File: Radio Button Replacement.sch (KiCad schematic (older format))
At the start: 19 parts, among them SW1 SW_Push_SPDT_1_3_2, SW2 SW_Push_SPDT_1_3_2, SW3 SW_Push_SPDT_1_3_2, SW4 SW_Push_SPDT_1_3_2

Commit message: Center marks added
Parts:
- L1: Description (none) -> None; Manufacturer Name (none) -> None; Manufacturer Part No. (none) -> None; Source (none) -> None
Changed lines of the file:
@@
 F 1 "Logo" H 7135 6255 50  0000 L CNN
 F 2 "Logos:OSHW-Logo2_7.3x6mm_SilkScreen" H 7050 6300 50  0001 C CNN
-F 3 "" H 7050 6300 50  0001 C CNN
+F 3 "None" H 7050 6300 50  0001 C CNN
+F 4 "None" H 7050 6300 50  0001 C CNN "Description"
+F 5 "None" H 7050 6300 50  0001 C CNN "Manufacturer Name"
+F 6 "None" H 7050 6300 50  0001 C CNN "Manufacturer Part No."
+F 7 "None" H 7050 6300 50  0001 C CNN "Source"
 	1    7050 6300
 	1    0    0    -1

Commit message: Update resistor sizes
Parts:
- R1, R2, R3, R4, R5, R6, R7, R8: footprint Resistor_THT:R_Axial_DIN0204_L3.6mm_D1.6mm_P5.08mm_Horizontal -> Resistor_THT:R_Axial_DIN0204_L3.6mm_D1.6mm_P7.62mm_Horizontal
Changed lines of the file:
@@
 F 0 "R1" V 5500 3100 50  0000 C CNN
 F 1 "2.2k" V 5700 3100 50  0000 C CNN
-F 2 "Resistor_THT:R_Axial_DIN0204_L3.6mm_D1.6mm_P5.08mm_Horizontal" V 5530 3100 50  0001 C CNN
+F 2 "Resistor_THT:R_Axial_DIN0204_L3.6mm_D1.6mm_P7.62mm_Horizontal" V 5530 3100 50  0001 C CNN
 F 3 "https://www.seielect.com/catalog/sei-rnf_rnmf.pdf" H 5600 3100 50  0001 C CNN
 F 4 "2.2 kOhms ±1% 0.25W, 1/4W Through Hole Resistor Axial Flame Retardant Coating, Safety Metal Film" H 5600 3100 50  0001 C CNN "Description"
@@
 F 0 "R4" V 7200 3200 50  0000 C CNN
 F 1 "2.2k" V 7400 3200 50  0000 C CNN
-F 2 "Resistor_THT:R_Axial_DIN0204_L3.6mm_D1.6mm_P5.08mm_Horizontal" V 7230 3200 50  0001 C CNN
+F 2 "Resistor_THT:R_Axial_DIN0204_L3.6mm_D1.6mm_P7.62mm_Horizontal" V 7230 3200 50  0001 C CNN
 F 3 "https://www.seielect.com/catalog/sei-rnf_rnmf.pdf" H 7300 3200 50  0001 C CNN
 F 4 "2.2 kOhms ±1% 0.25W, 1/4W Through Hole Resistor Axial Flame Retardant Coating, Safety Metal Film" H 7300 3200 50  0001 C CNN "Description"
@@
 F 0 "R2" V 6050 2550 50  0000 C CNN
 F 1 "2.2k" V 6250 2550 50  0000 C CNN
-F 2 "Resistor_THT:R_Axial_DIN0204_L3.6mm_D1.6mm_P5.08mm_Horizontal" V 6080 2550 50  0001 C CNN
+F 2 "Resistor_THT:R_Axial_DIN0204_L3.6mm_D1.6mm_P7.62mm_Horizontal" V 6080 2550 50  0001 C CNN
 F 3 "https://www.seielect.com/catalog/sei-rnf_rnmf.pdf" H 6150 2550 50  0001 C CNN
 F 4 "2.2 kOhms ±1% 0.25W, 1/4W Through Hole Resistor Axial Flame Retardant Coating, Safety Metal Film" H 6150 2550 50  0001 C CNN "Description"
@@
 F 0 "R3" V 6650 2550 50  0000 C CNN
 F 1 "2.2k" V 6850 2550 50  0000 C CNN
-F 2 "Resistor_THT:R_Axial_DIN0204_L3.6mm_D1.6mm_P5.08mm_Horizontal" V 6680 2550 50  0001 C CNN
+F 2 "Resistor_THT:R_Axial_DIN0204_L3.6mm_D1.6mm_P7.62mm_Horizontal" V 6680 2550 50  0001 C CNN
 F 3 "https://www.seielect.com/catalog/sei-rnf_rnmf.pdf" H 6750 2550 50  0001 C CNN
 F 4 "2.2 kOhms ±1% 0.25W, 1/4W Through Hole Resistor Axial Flame Retardant Coating, Safety Metal Film" H 6750 2550 50  0001 C CNN "Description"
@@
 F 0 "R5" V 5500 4550 50  0000 C CNN
 F 1 "2.2k" V 5700 4550 50  0000 C CNN
-F 2 "Resistor_THT:R_Axial_DIN0204_L3.6mm_D1.6mm_P5.08mm_Horizontal" V 5530 4550 50  0001 C CNN
+F 2 "Resistor_THT:R_Axial_DIN0204_L3.6mm_D1.6mm_P7.62mm_Horizontal" V 5530 4550 50  0001 C CNN
 F 3 "https://www.seielect.com/catalog/sei-rnf_rnmf.pdf" H 5600 4550 50  0001 C CNN
 F 4 "2.2 kOhms ±1% 0.25W, 1/4W Through Hole Resistor Axial Flame Retardant Coating, Safety Metal Film" H 5600 4550 50  0001 C CNN "Description"
@@
 F 0 "R8" V 7200 4650 50  0000 C CNN
 F 1 "2.2k" V 7400 4650 50  0000 C CNN
-F 2 "Resistor_THT:R_Axial_DIN0204_L3.6mm_D1.6mm_P5.08mm_Horizontal" V 7230 4650 50  0001 C CNN
+F 2 "Resistor_THT:R_Axial_DIN0204_L3.6mm_D1.6mm_P7.62mm_Horizontal" V 7230 4650 50  0001 C CNN
 F 3 "https://www.seielect.com/catalog/sei-rnf_rnmf.pdf" H 7300 4650 50  0001 C CNN
 F 4 "2.2 kOhms ±1% 0.25W, 1/4W Through Hole Resistor Axial Flame Retardant Coating, Safety Metal Film" H 7300 4650 50  0001 C CNN "Description"
@@
 F 0 "R6" V 6050 4000 50  0000 C CNN
 F 1 "2.2k" V 6250 4000 50  0000 C CNN
-F 2 "Resistor_THT:R_Axial_DIN0204_L3.6mm_D1.6mm_P5.08mm_Horizontal" V 6080 4000 50  0001 C CNN
+F 2 "Resistor_THT:R_Axial_DIN0204_L3.6mm_D1.6mm_P7.62mm_Horizontal" V 6080 4000 50  0001 C CNN
 F 3 "https://www.seielect.com/catalog/sei-rnf_rnmf.pdf" H 6150 4000 50  0001 C CNN
 F 4 "2.2 kOhms ±1% 0.25W, 1/4W Through Hole Resistor Axial Flame Retardant Coating, Safety Metal Film" H 6150 4000 50  0001 C CNN "Description"
@@
 F 0 "R7" V 6650 4000 50  0000 C CNN
 F 1 "2.2k" V 6850 4000 50  0000 C CNN
-F 2 "Resistor_THT:R_Axial_DIN0204_L3.6mm_D1.6mm_P5.08mm_Horizontal" V 6680 4000 50  0001 C CNN
+F 2 "Resistor_THT:R_Axial_DIN0204_L3.6mm_D1.6mm_P7.62mm_Horizontal" V 6680 4000 50  0001 C CNN
 F 3 "https://www.seielect.com/catalog/sei-rnf_rnmf.pdf" H 6750 4000 50  0001 C CNN
 F 4 "2.2 kOhms ±1% 0.25W, 1/4W Through Hole Resistor Axial Flame Retardant Coating, Safety Metal Film" H 6750 4000 50  0001 C CNN "Description"

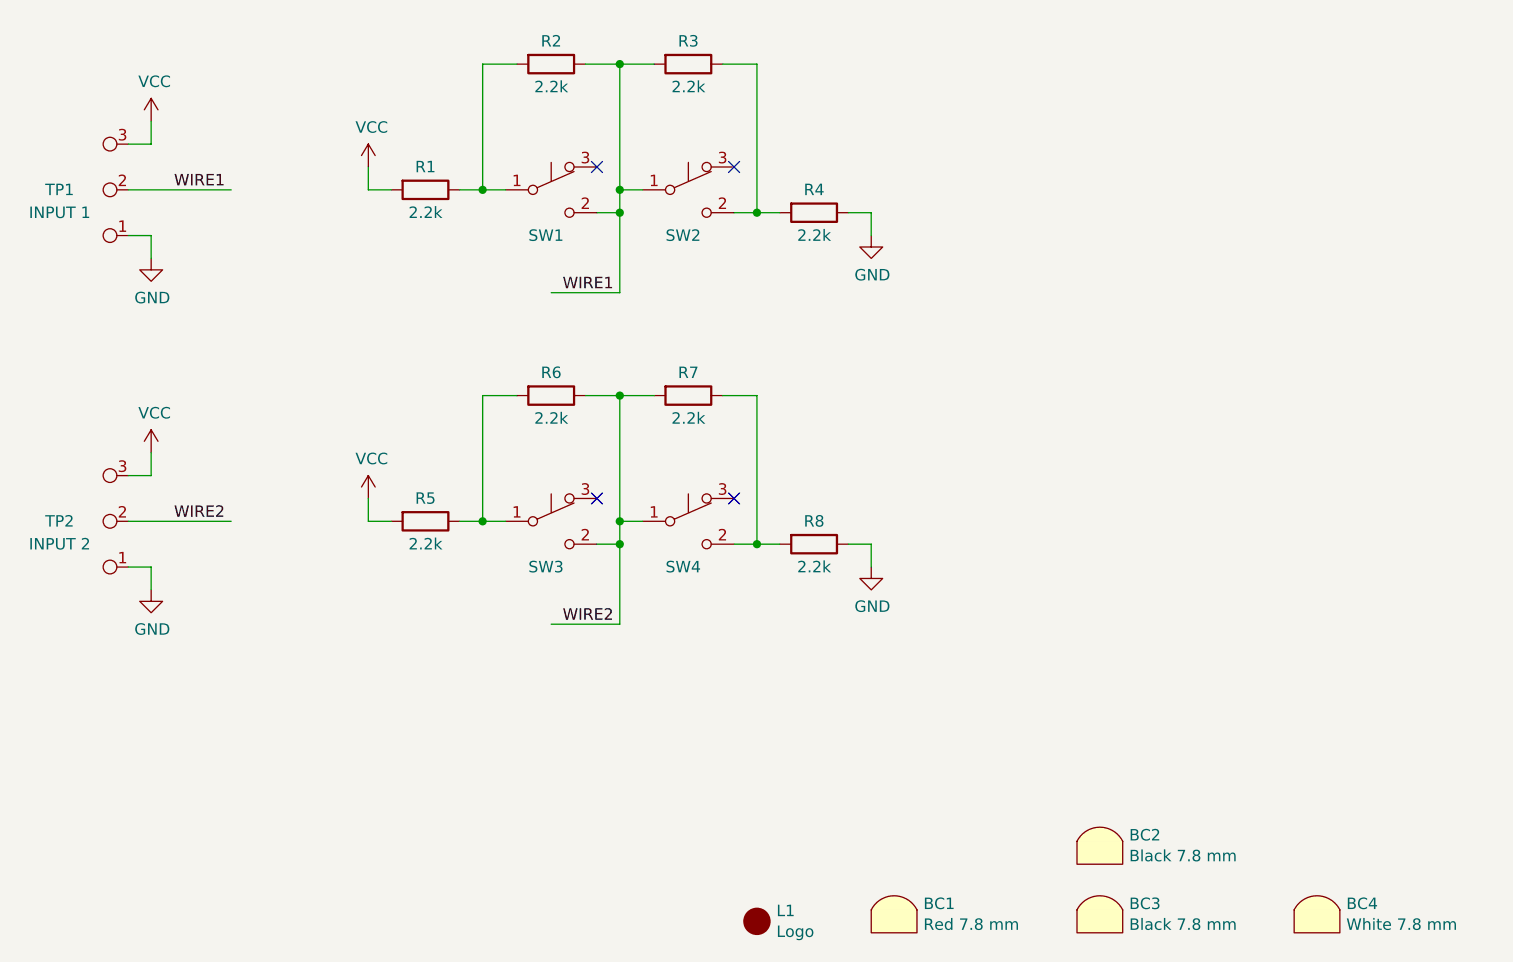
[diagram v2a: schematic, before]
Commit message: Renumbering of components, PCB updates
Renumbering of components, PCB updates
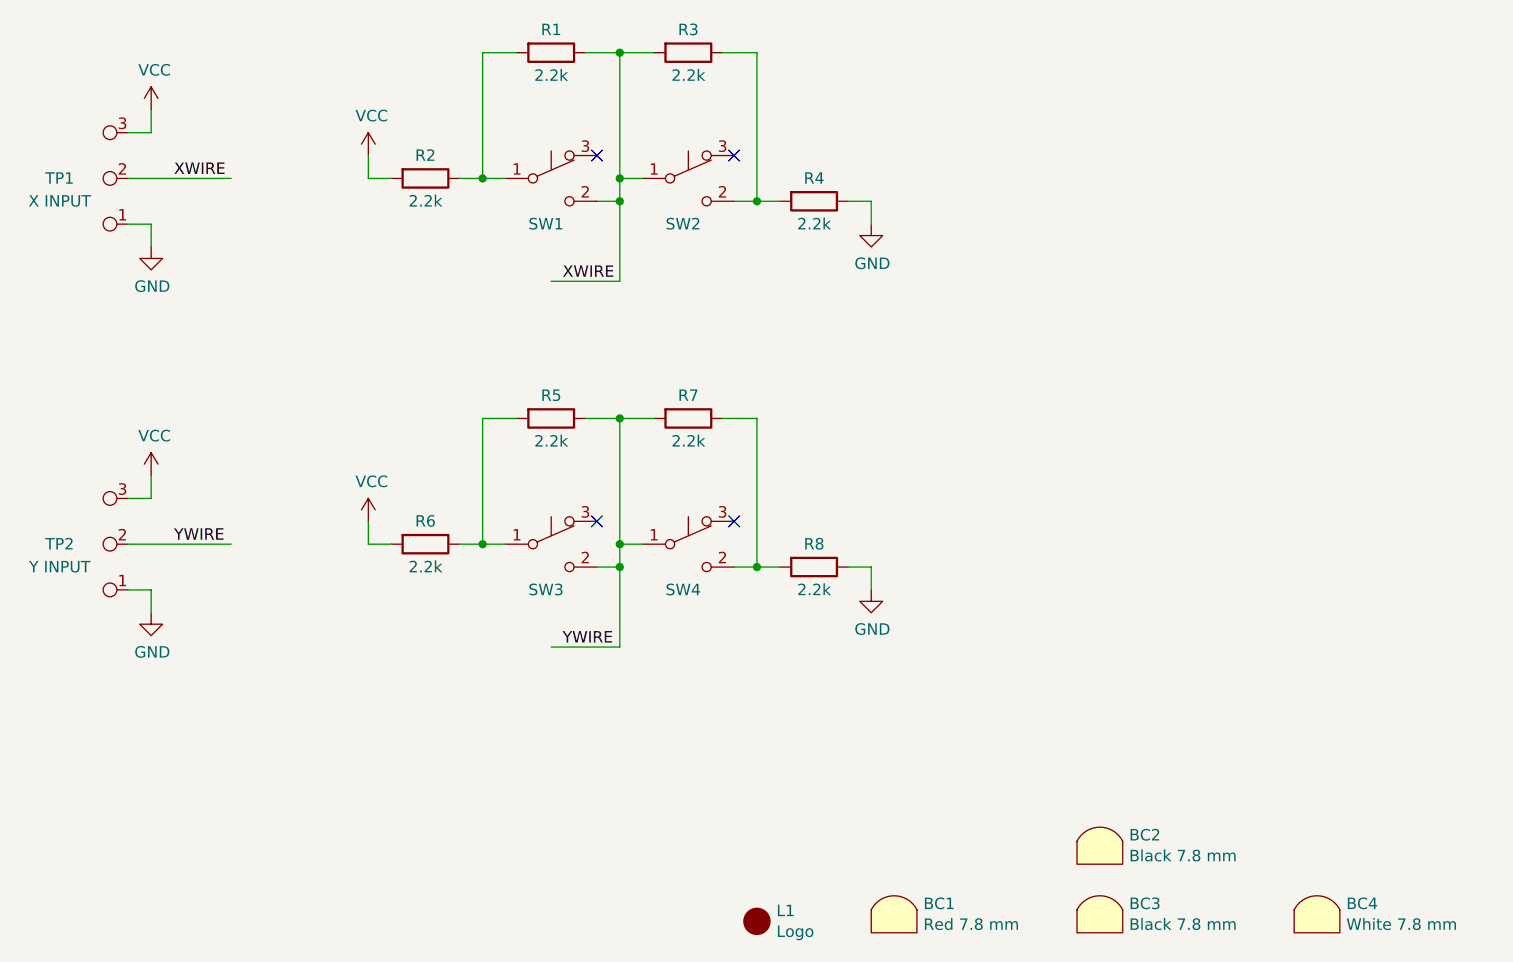
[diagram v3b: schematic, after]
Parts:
- TP1: renamed from TP2; Name INPUT 2 -> X INPUT
- TP2: renamed from TP1; Name INPUT 1 -> Y INPUT
- renumbered R6 to R1, R5 to R2, R7 to R3, R8 to R4, R2 to R5, R1 to R6, R3 to R7, R4 to R8, SW3 to SW1, SW4 to SW2, SW1 to SW3, SW2 to SW4
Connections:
- net labels added: XWIRE, YWIRE
- net labels removed: WIRE1, WIRE2
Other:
- moved on the sheet: R1, R2, R3, R4, R5, R6, R7, R8, SW1, SW2, SW3, SW4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
